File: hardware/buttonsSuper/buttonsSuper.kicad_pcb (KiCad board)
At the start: 2 copper layers, 137.2 x 76.5 mm, 21 parts, among them P1 5034801000

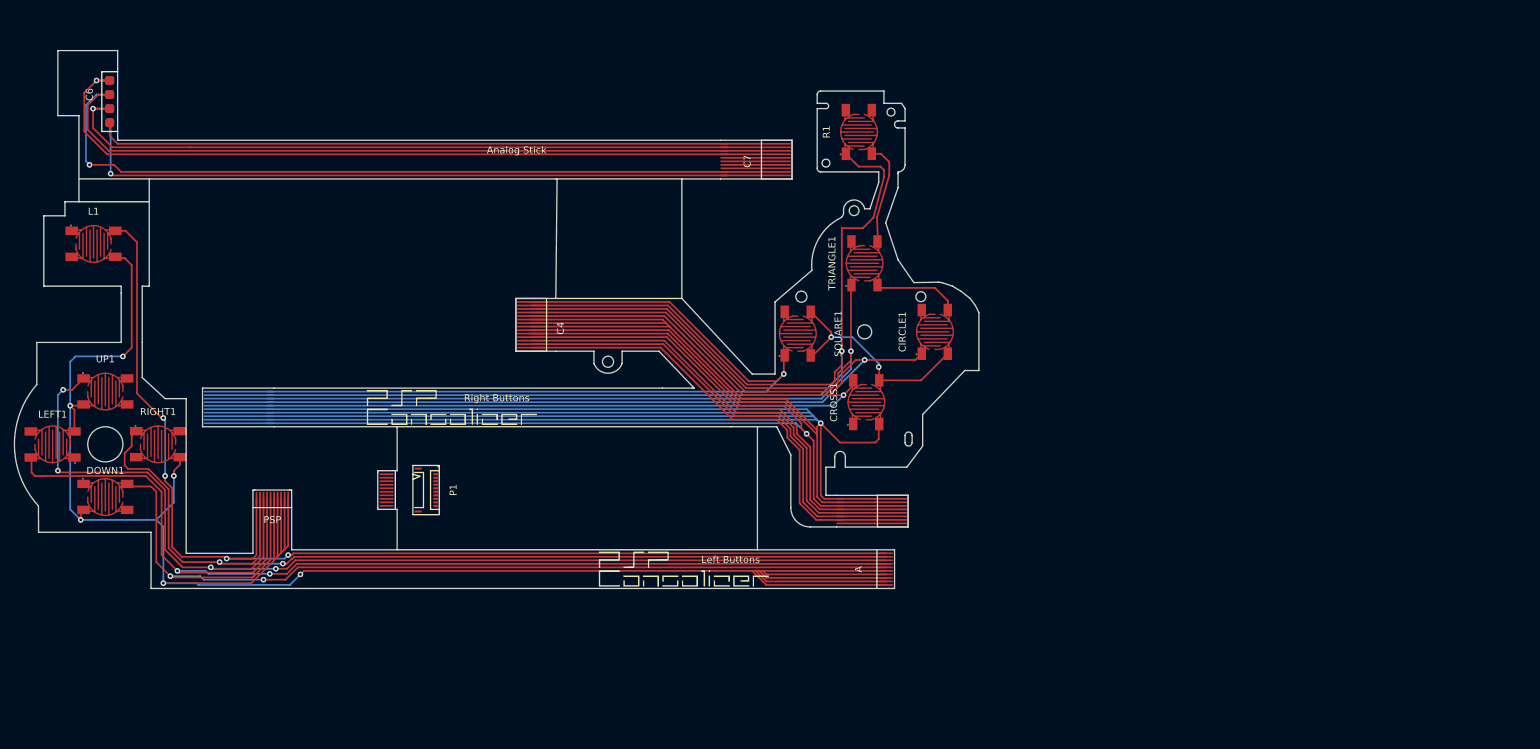
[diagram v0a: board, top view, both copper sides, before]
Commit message: wip
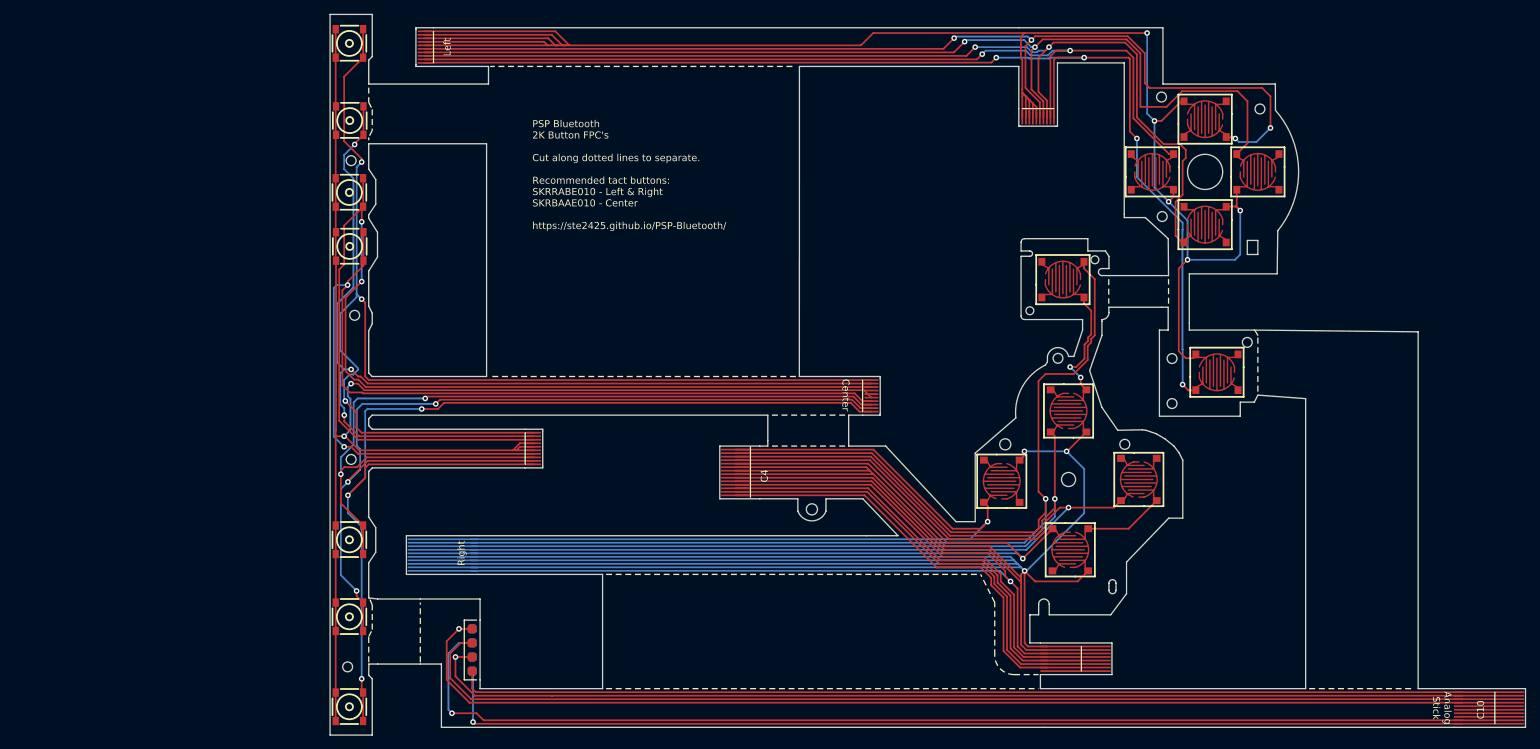
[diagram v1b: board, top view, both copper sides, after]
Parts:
- removed C7: flex-conector_10, consolizer:flex_long_10
- removed CIRCLE1, CROSS1, R1, SQUARE1, TRIANGLE1: K2-1187SQ-E4SW-06, JLCPCB_footprint:KEY-SMD_4P-L5.2-W5.2-P3.70-LS6.4_1
- removed G*** (x2): LOGO, consolizer:logo_small
- removed P1: 5034801000, JLCPCB_footprint:FPC-SMD_5034801000
- added C10: flex-conector_10, consolizer:flex_long_10, F.Cu at (247.3, 148.0)
- added C9: flex-conector_10, consolizer:flex_short_10, F.Cu at (158.5, 103.6)
- added L2: SKRRABE010, JLCPCB_footprint:KEY-SMD_4P-L5.2-W5.2-P3.70-LS6.4_1, F.Cu at (186.8, 125.2)
- added L3: SKRRABE010, JLCPCB_footprint:KEY-SMD_4P-L5.2-W5.2-P3.70-LS6.4_1, F.Cu at (185.7, 86.8)
- added L4: SKRRABE010, JLCPCB_footprint:KEY-SMD_4P-L5.2-W5.2-P3.70-LS6.4_1, F.Cu at (186.5, 105.5)
- added L5: SKRRABE010, JLCPCB_footprint:KEY-SMD_4P-L5.2-W5.2-P3.70-LS6.4_1, F.Cu at (177.0, 115.5)
- added L6: SKRRABE010, JLCPCB_footprint:KEY-SMD_4P-L5.2-W5.2-P3.70-LS6.4_1, F.Cu at (196.5, 115.2)
- added U1: SKRBAAE010, JLCPCB_footprint:KEY-SMD_4P-L4.8-W4.8-P3.65_SKRBAAE010, F.Cu at (84.2, 74.4)
- added U2: SKRBAAE010, JLCPCB_footprint:KEY-SMD_4P-L4.8-W4.8-P3.65_SKRBAAE010, F.Cu at (84.3, 82.1)
- added U3: SKRBAAE010, JLCPCB_footprint:KEY-SMD_4P-L4.8-W4.8-P3.65_SKRBAAE010, F.Cu at (84.2, 53.2)
- added U4: SKRBAAE010, JLCPCB_footprint:KEY-SMD_4P-L4.8-W4.8-P3.65_SKRBAAE010, F.Cu at (84.3, 64.2)
- added U5: SKRBAAE010, JLCPCB_footprint:KEY-SMD_4P-L4.8-W4.8-P3.65_SKRBAAE010, F.Cu at (84.2, 123.8)
- added U6: SKRBAAE010, JLCPCB_footprint:KEY-SMD_4P-L4.8-W4.8-P3.65_SKRBAAE010, F.Cu at (84.2, 134.8)
- added U7: SKRBAAE010, JLCPCB_footprint:KEY-SMD_4P-L4.8-W4.8-P3.65_SKRBAAE010, F.Cu at (84.2, 147.6)
- DOWN1, L1, LEFT1, RIGHT1, UP1: value K2-1187SQ-E4SW-06 -> SKRRABE010
- moved LEFT1 175.8 mm to (213.4, 71.5), turned to 0 degrees
- moved DOWN1 165.4 mm to (205.9, 64.0), turned to 180 degrees
- moved L1 160.8 mm to (207.6, 100.0), turned to 180 degrees
- moved UP1 158.2 mm to (205.9, 79.0), turned to 180 degrees
- moved RIGHT1 146.6 mm to (198.4, 71.5)
- moved C2 121.2 mm to (181.9, 63.7), turned to 180 degrees
- moved C1 99.4 mm to (94.9, 53.5), turned to 90 degrees
- moved C6 93.5 mm to (101.8, 138.7)
- moved C3 35.8 mm to (179.4, 138.5)
- moved C5 35.8 mm to (96.5, 126.2)
- moved C4 35.8 mm to (139.1, 114.1)
- moved C8 21.6 mm to (110.5, 111.1), turned to -90 degrees
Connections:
- C6 pad 1: GND -> /gnd3
- C6 pad 2: /X_1 -> /analog_x
- C6 pad 4: /Y_1 -> /Analog_y
- C6 pad 5: GND -> /gnd3
- C6 pad 6: /X_2 -> /PSP_x
- C6 pad 8: /Y_2 -> /PSP_y
- C8 pad 1: Net-(C8-Pad1) -> /start
- C8 pad 10: Net-(C8-Pad10) -> /home
- C8 pad 2: Net-(C8-Pad2) -> /select
- C8 pad 3: Net-(C8-Pad3) -> /music
- C8 pad 4: Net-(C8-Pad4) -> /gnd2
- C8 pad 5: Net-(C8-Pad5) -> /gnd2
- C8 pad 6: Net-(C8-Pad6) -> /gnd2
- C8 pad 7: Net-(C8-Pad7) -> /screen
- C8 pad 8: Net-(C8-Pad8) -> /vol up
- C8 pad 9: Net-(C8-Pad9) -> /vol down
- DOWN1 pad 2: /down -> GND
- L1 pad 2: /l1 -> GND
- LEFT1 pad 2: /left -> GND
- RIGHT1 pad 2: /right -> GND
- UP1 pad 2: /up -> GND
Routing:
- net /gnd2: track 0.00 -> 216.6 mm, vias 0 -> 2
- net /start: track 0.00 -> 173.0 mm, vias 0 -> 3
- net /music: track 0.00 -> 164.9 mm, vias 0 -> 2
- net /gnd3: track 0.00 -> 157.6 mm, vias 0 -> 1
- net /PSP_x: track 0.00 -> 156.9 mm, vias 0 -> 1
- net /analog_x: track 0.00 -> 152.5 mm
- net /select: track 0.00 -> 152.0 mm, vias 0 -> 3
- net /screen: track 0.00 -> 151.9 mm, vias 0 -> 2
- net /PSP_y: track 0.00 -> 148.2 mm, vias 0 -> 1
- net /home: track 0.00 -> 148.1 mm, vias 0 -> 3
- net /Analog_y: track 0.00 -> 143.6 mm
- net GND: track 427.9 -> 286.4 mm, vias 7 -> 5
- net /vol down: track 0.00 -> 136.2 mm, vias 0 -> 3
- net /vol up: track 0.00 -> 126.8 mm, vias 0 -> 2
- net /X_2: track 103.9 -> 0.00 mm, vias 1 -> 0
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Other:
- board size 137.2 x 76.5 mm -> 159.9 x 102.5 mm
- board text added: "Center"
- board text added: "Left"
- board text added: "PSP Bluetooth 2K Button FPC's Cut along dotted lines to separate. Recommended tact buttons: SKRRABE010 - Left & Right SKRBAAE010 - Center https://ste2425.github.io/PSP-Bluetooth/"
- board text added: "Right"
- board text added: "Stiffener: Polyimide Stiffener thickness: 0.2mm Stiffener Location: Refer to User.Drawings layer This is intended to be manufactured as a single board, not as multiple individual boards. Thanks :)"
- board text removed: "A"
- board text removed: "B"
- board text removed: "Left Buttons"
- board text removed: "PSP"
- board text removed: "Right Buttons"
